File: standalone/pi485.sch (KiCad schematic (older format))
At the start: 29 parts, among them J1 RS485, P1 Rasperry Pi, P2 PWR, P3 TERM, P4 RO, Q1 2N3904, Q2 2N3904, Q3 2N3904, Q4 2N3906, U1 NE555, U2 MAX485

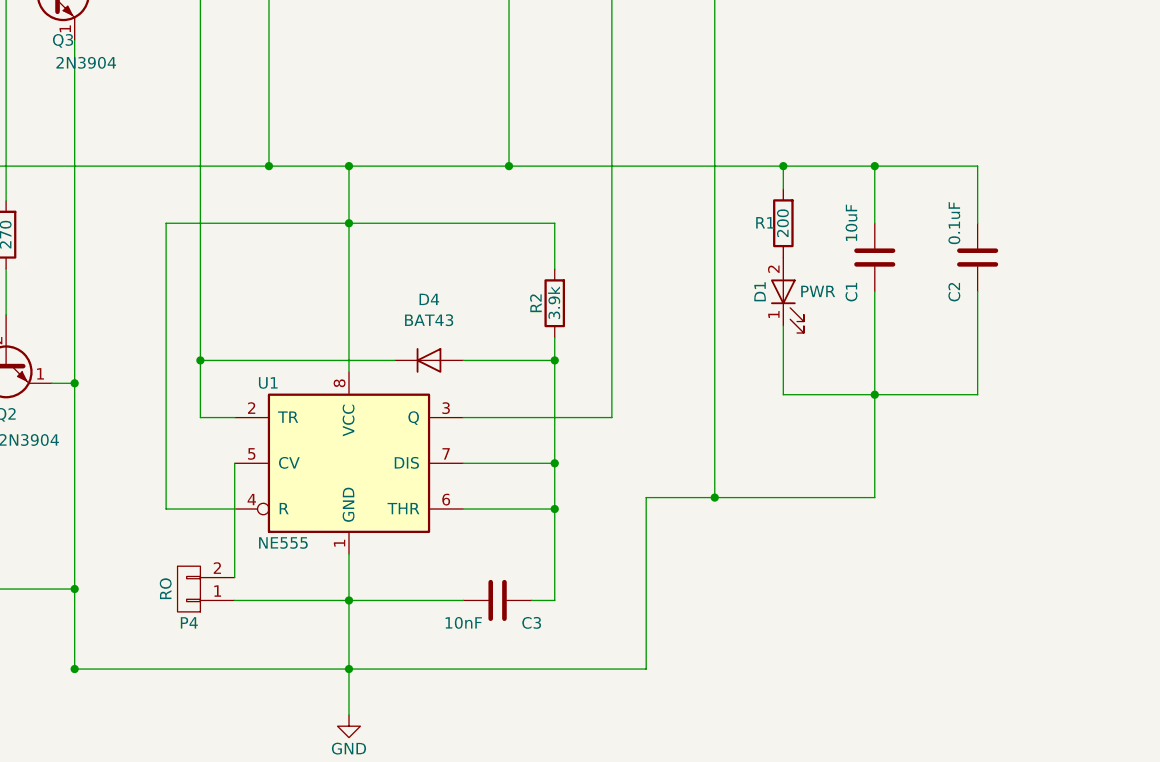
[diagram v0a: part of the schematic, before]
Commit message: Esthetics and what-not...
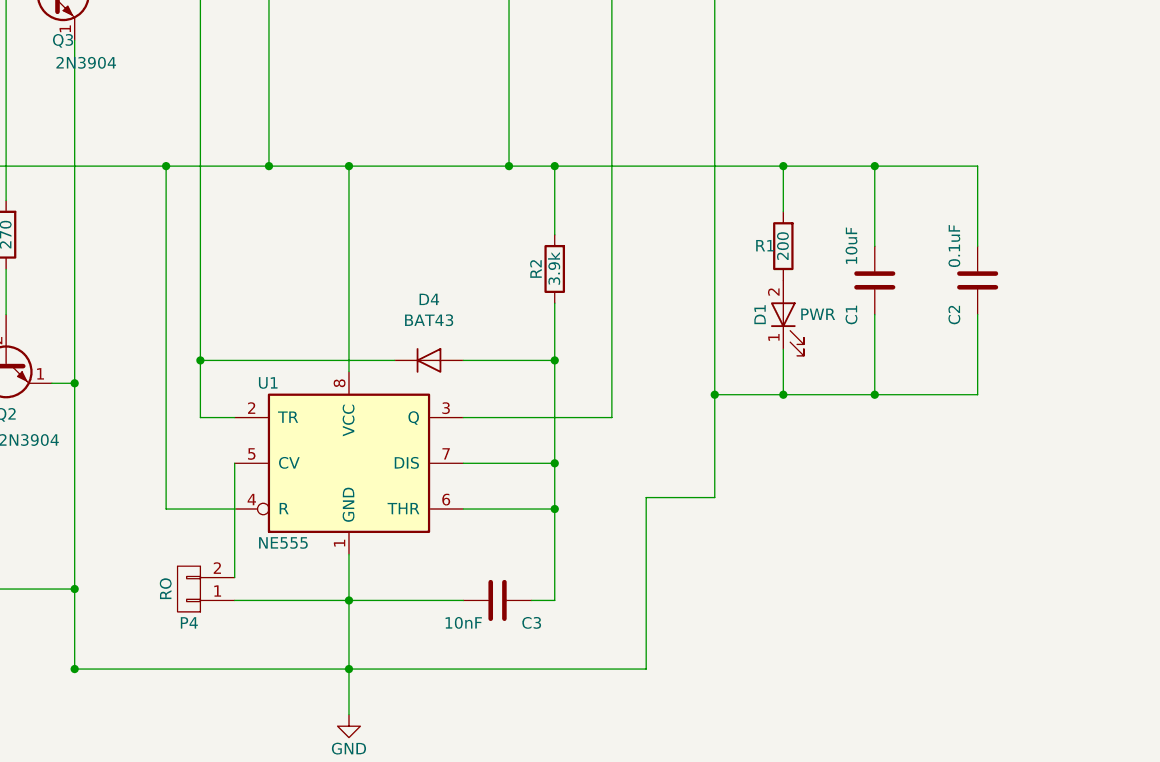
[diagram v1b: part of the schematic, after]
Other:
- moved on the sheet: C1, C2, D1, R1, R2
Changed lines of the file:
@@
 L R R1
 U 1 1 586E84C4
-P 7400 4800
-F 0 "R1" H 7480 4800 50  0000 C CNN
-F 1 "200" V 7400 4800 50  0000 C CNN
-F 2 "Resistors_THT:Resistor_Horizontal_RM10mm" V 7550 4100 50  0001 C CNN
-F 3 "" H 7400 4800 50  0000 C CNN
-	1    7400 4800
+P 7400 4900
+F 0 "R1" H 7480 4900 50  0000 C CNN
+F 1 "200" V 7400 4900 50  0000 C CNN
+F 2 "Resistors_THT:Resistor_Horizontal_RM10mm" V 7550 4200 50  0001 C CNN
+F 3 "" H 7400 4900 50  0000 C CNN
+	1    7400 4900
 	-1   0    0    1
 $EndComp
@@
 L LED D1
 U 1 1 586E8531
-P 7400 5100
-F 0 "D1" H 7400 5200 50  0000 C CNN
-F 1 "PWR" V 7400 4950 50  0000 C CNN
-F 2 "LEDs:LED-3MM" H 7350 4900 50  0001 C CNN
-F 3 "" H 7400 5100 50  0000 C CNN
-	1    7400 5100
+P 7400 5200
+F 0 "D1" H 7400 5300 50  0000 C CNN
+F 1 "PWR" V 7400 5050 50  0000 C CNN
+F 2 "LEDs:LED-3MM" H 7350 5000 50  0001 C CNN
+F 3 "" H 7400 5200 50  0000 C CNN
+	1    7400 5200
 	0    -1   -1   0
 $EndComp
@@
 L R R2
 U 1 1 586E88D3
-P 6400 5150
-F 0 "R2" V 6480 5150 50  0000 C CNN
-F 1 "3.9k" V 6400 5150 50  0000 C CNN
-F 2 "Resistors_THT:Resistor_Horizontal_RM10mm" H 5500 5150 50  0001 C CNN
-F 3 "" H 6400 5150 50  0000 C CNN
-	1    6400 5150
+P 6400 5000
+F 0 "R2" V 6480 5000 50  0000 C CNN
+F 1 "3.9k" V 6400 5000 50  0000 C CNN
+F 2 "Resistors_THT:Resistor_Horizontal_RM10mm" H 5500 5000 50  0001 C CNN
+F 3 "" H 6400 5000 50  0000 C CNN
+	1    6400 5000
 	-1   0    0    1
 $EndComp
@@
 L C C2
 U 1 1 5876F3DF
-P 8250 4950
-F 0 "C2" V 8350 5100 50  0000 C CNN
-F 1 "0.1uF" V 8350 4800 50  0000 C CNN
-F 2 "Capacitors_THT:C_Rect_L7_W2.5_P5" V 8450 4650 50  0001 C CNN
-F 3 "" H 8250 4950 50  0000 C CNN
-	1    8250 4950
+P 8250 5050
+F 0 "C2" V 8350 5200 50  0000 C CNN
+F 1 "0.1uF" V 8350 4900 50  0000 C CNN
+F 2 "Capacitors_THT:C_Rect_L7_W2.5_P5" V 8450 4750 50  0001 C CNN
+F 3 "" H 8250 5050 50  0000 C CNN
+	1    8250 5050
 	-1   0    0    1
 $EndComp
@@
 L C C1
 U 1 1 5876F5F2
-P 7800 4950
-F 0 "C1" V 7900 5100 50  0000 C CNN
-F 1 "10uF" V 7900 4800 50  0000 C CNN
-F 2 "Capacitors_THT:C_Radial_D5_L11_P2" V 8000 4650 50  0001 C CNN
-F 3 "" H 7800 4950 50  0000 C CNN
-	1    7800 4950
+P 7800 5050
+F 0 "C1" V 7900 5200 50  0000 C CNN
+F 1 "10uF" V 7900 4900 50  0000 C CNN
+F 2 "Capacitors_THT:C_Radial_D5_L11_P2" V 8000 4750 50  0001 C CNN
+F 3 "" H 7800 5050 50  0000 C CNN
+	1    7800 5050
 	-1   0    0    1
 $EndComp
@@
 	5500 4550 5500 5450
 Wire Wire Line
-	6400 5300 6400 6450
+	6400 5150 6400 6450
 Wire Wire Line
 	6400 5850 6000 5850
@@
 	5000 6050 4700 6050
 Wire Wire Line
-	4700 6050 4700 4800
-Connection ~ 5500 4800
+	4700 6050 4700 4550
 Wire Wire Line
 	2150 2800 5150 2800
@@
 Connection ~ 2600 2900
 Wire Wire Line
-	4700 4800 6400 4800
-Wire Wire Line
-	6400 4800 6400 5000
+	6400 4550 6400 4850
 Wire Wire Line
 	5700 5400 4850 5400
@@
 	5000 6350 5000 5850
 Wire Wire Line
-	7400 4550 7400 4650
-Wire Wire Line
-	7800 6000 7800 5100
-Wire Wire Line
-	8250 5550 8250 5100
-Wire Wire Line
-	8250 4550 8250 4800
-Wire Wire Line
-	7800 4550 7800 4800
+	7400 4550 7400 4750
+Wire Wire Line
+	8250 5550 8250 5200
+Wire Wire Line
+	8250 4550 8250 4900
+Wire Wire Line
+	7800 4550 7800 4900
 Connection ~ 7800 4550
 Connection ~ 7800 5550
@@
 Wire Wire Line
 	4300 6750 6800 6750
-Wire Wire Line
-	6800 6000 7800 6000
 Connection ~ 5500 6750
 Wire Wire Line
@@
 	6200 2100 6200 4550
 Wire Wire Line
-	7400 5550 8250 5550
+	7100 5550 8250 5550
 Connection ~ 6200 4550
 Connection ~ 7400 4550
 Wire Wire Line
-	7400 5550 7400 5250
+	7400 5550 7400 5350
 Wire Wire Line
 	2900 3800 2900 2150
-Connection ~ 7100 6000
 Wire Wire Line
 	2250 4550 8250 4550
@@
 Wire Wire Line
 	5150 2800 5150 3300
+Connection ~ 6400 4550
+Connection ~ 4700 4550
+Connection ~ 7100 5550
+Connection ~ 7400 5550
+Wire Wire Line
+	6800 6000 7100 6000
+Wire Wire Line
+	7800 5200 7800 5550
 $EndSCHEMATC
